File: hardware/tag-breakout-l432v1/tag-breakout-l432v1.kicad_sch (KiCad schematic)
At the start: 29 parts, among them J1 Conn_01x04_Female, J102 Conn_02x05_Odd_Even, J104 USB_B_Mini, J2 Conn_01x02_Male, SW1 SW_DIP_x04, U1 XC6206, U101 STM32F042K6Tx, U105 Tactile Switch, U2 TS5A3159ADBVR, U4 TS5A3159ADBVR

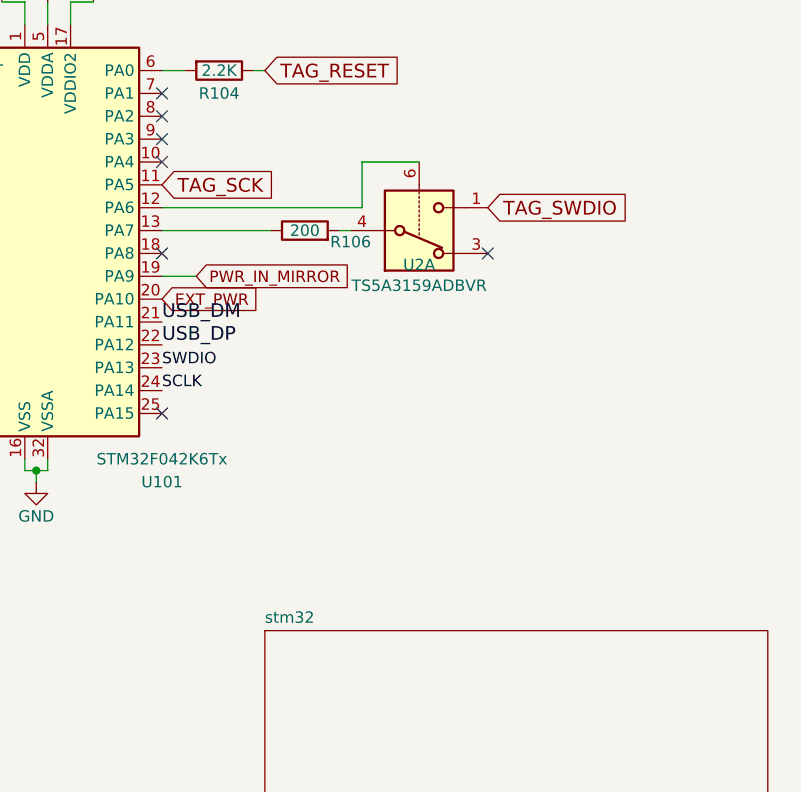
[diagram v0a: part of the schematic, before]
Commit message: update proto boards
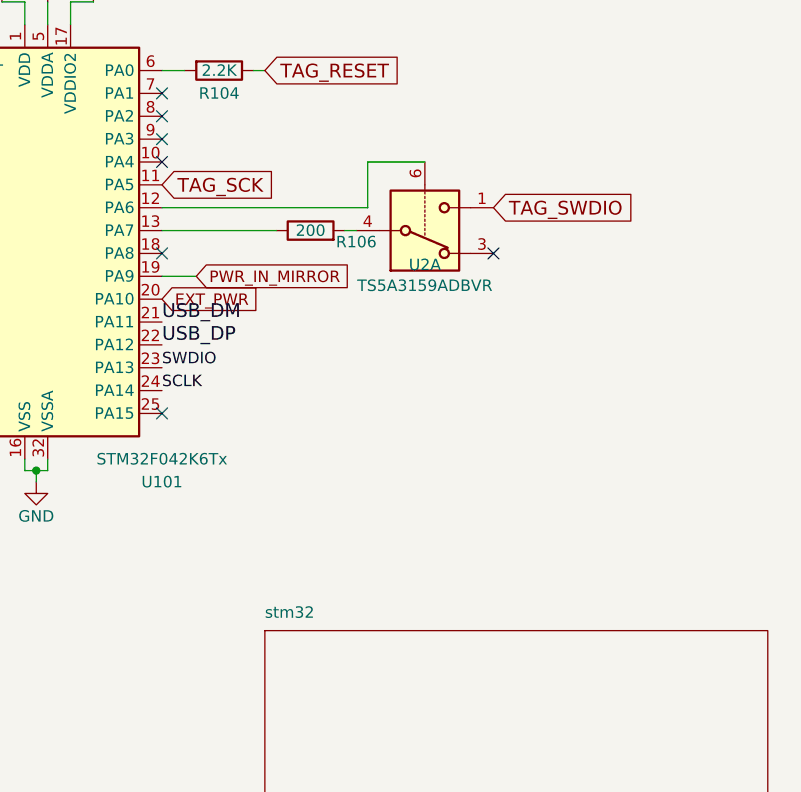
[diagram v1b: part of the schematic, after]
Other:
- moved on the sheet: R106, U2A
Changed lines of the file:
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@@
 	)
 	(no_connect
-		(at 220.345 97.79)
+		(at 220.98 97.79)
 	)
 	(no_connect
@@
 	(wire
 		(pts
-			(xy 206.375 87.63) (xy 212.725 87.63)
+			(xy 207.01 87.63) (xy 213.36 87.63)
 		)
 		(stroke
@@
 	(wire
 		(pts
-			(xy 203.835 95.25) (xy 205.105 95.25)
+			(xy 204.47 95.25) (xy 205.74 95.25)
 		)
 		(stroke
@@
 	(wire
 		(pts
-			(xy 206.375 87.63) (xy 206.375 92.71)
+			(xy 207.01 87.63) (xy 207.01 92.71)
 		)
 		(stroke
@@
 	(wire
 		(pts
-			(xy 184.15 95.25) (xy 196.215 95.25)
+			(xy 184.15 95.25) (xy 196.85 95.25)
 		)
 		(stroke
@@
 	(wire
 		(pts
-			(xy 184.15 92.71) (xy 206.375 92.71)
+			(xy 184.15 92.71) (xy 207.01 92.71)
 		)
 		(stroke
@@
 	(global_label "TAG_SWDIO"
 		(shape input)
-		(at 220.345 92.71 0)
+		(at 220.98 92.71 0)
 		(fields_autoplaced yes)
 		(effects
@@
 		)
 		(property "Intersheetrefs" "${INTERSHEET_REFS}"
-			(at 235.3337 92.71 0)
+			(at 235.9687 92.71 0)
 			(effects
 				(font
@@
 	(symbol
 		(lib_id "Device:R")
-		(at 200.025 95.25 90)
+		(at 200.66 95.25 90)
 		(unit 1)
 		(exclude_from_sim no)
@@
 		(dnp no)
 		(property "Reference" "R106"
-			(at 205.105 96.52 90)
+			(at 205.74 96.52 90)
 			(effects
 				(font
@@
 		)
 		(property "Value" "200"
-			(at 200.025 95.25 90)
+			(at 200.66 95.25 90)
 			(effects
 				(font
@@
 		)
 		(property "Footprint" "Resistor_SMD:R_0603_1608Metric"
-			(at 200.025 97.028 90)
+			(at 200.66 97.028 90)
 			(effects
 				(font
@@
 		)
 		(property "Datasheet" ""
-			(at 200.025 95.25 0)
+			(at 200.66 95.25 0)
 			(effects
 				(font
@@
 		)
 		(property "Description" ""
-			(at 200.025 95.25 0)
+			(at 200.66 95.25 0)
 			(effects
 				(font
@@
 		)
 		(property "LCSC" "C8218 "
-			(at 296.545 187.96 0)
+			(at 297.18 187.96 0)
 			(effects
 				(font
@@
 		)
 		(property "MFN" "Uniroyal Elec."
-			(at 296.545 187.96 0)
+			(at 297.18 187.96 0)
 			(effects
 				(font
@@
 		)
 		(property "MPN" "0603WAF1000T5E"
-			(at 296.545 187.96 0)
+			(at 297.18 187.96 0)
 			(effects
 				(font
@@
 		)
 		(property "Digikey" ""
-			(at 200.025 95.25 0)
+			(at 200.66 95.25 0)
 			(effects
 				(font
@@
 	(symbol
 		(lib_id "Analog_Switch:TS5A3159ADBVR")
-		(at 212.725 95.25 0)
+		(at 213.36 95.25 0)
 		(mirror x)
 		(unit 1)
@@
 		(dnp no)
 		(property "Reference" "U2"
-			(at 212.725 99.06 0)
+			(at 213.36 99.06 0)
 			(effects
 				(font
@@
 		)
 		(property "Value" "TS5A3159ADBVR"
-			(at 212.725 101.3714 0)
+			(at 213.36 101.3714 0)
 			(effects
 				(font
@@
 		)
 		(property "Footprint" "Package_TO_SOT_SMD:SOT-23-6"
-			(at 212.725 87.63 0)
+			(at 213.36 87.63 0)
 			(effects
 				(font
@@
 		)
 		(property "Datasheet" "http://www.ti.com/lit/ds/symlink/ts5a3159a.pdf"
-			(at 212.725 95.25 0)
+			(at 213.36 95.25 0)
 			(effects
 				(font
@@
 		)
 		(property "Description" "Single SPDT Analog Switch, 1.65-V to 5.5-V Single-Supply Operation, 1Ohm Ron, SOT-23-6"
-			(at 212.725 95.25 0)
+			(at 213.36 95.25 0)
 			(effects
 				(font
@@
 		)
 		(property "MFN" "TI"
-			(at 212.725 95.25 0)
+			(at 213.36 95.25 0)
 			(effects
 				(font
@@
 		)
 		(property "MPN" "TS5A3159ADBVR"
-			(at 212.725 95.25 0)
+			(at 213.36 95.25 0)
 			(effects
 				(font
@@
 		)
 		(property "LCSC" "C128405"
-			(at 212.725 95.25 0)
+			(at 213.36 95.25 0)
 			(effects
 				(font
@@
 		)
 		(property "Digikey" ""
-			(at 212.725 95.25 0)
+			(at 213.36 95.25 0)
 			(effects
 				(font
@@
 			)
 		)
-		(property "Datasheet" ""
+		(property "Datasheet" "~"
 			(at 60.96 171.45 0)
 			(effects
@@
 			)
 		)
-		(property "Description" "CONN RCPT USB2.0 MINI B SMD R/A"
+		(property "Description" "USB Mini Type B connector"
 			(at 57.15 170.18 0)
 			(effects
@@
 		(at 195.58 139.7)
 		(size 55.88 22.86)
-		(fields_autoplaced yes)
 		(stroke
 			(width 0)
@@
 		)
 		(property "Sheetname" "stm32"
-			(at 195.58 138.9884 0)
+			(at 195.58 138.43 0)
 			(effects
 				(font
